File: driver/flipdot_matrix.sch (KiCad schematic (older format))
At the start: 45 parts, among them J2 CONN_02X32, Q1 DUAL_NPN_MOSFET, Q10 DUAL_NPN_MOSFET, Q11 DUAL_NPN_MOSFET, Q12 DUAL_NPN_MOSFET, Q13 DUAL_NPN_MOSFET, Q14 DUAL_NPN_MOSFET, Q15 DUAL_NPN_MOSFET, Q16 DUAL_NPN_MOSFET, Q17 DUAL_NPN_MOSFET, Q18 DUAL_NPN_MOSFET, Q19 DUAL_NPN_MOSFET, Q2 DUAL_NPN_MOSFET, Q20 DUAL_NPN_MOSFET, Q21 DUAL_NPN_MOSFET, Q22 DUAL_NPN_MOSFET, Q23 DUAL_NPN_MOSFET, Q24 DUAL_NPN_MOSFET, Q25 DUAL_NPN_MOSFET, Q26 DUAL_NPN_MOSFET, Q27 DUAL_NPN_MOSFET, Q28 DUAL_NPN_MOSFET, Q29 DUAL_NPN_MOSFET, Q3 DUAL_NPN_MOSFET, Q30 DUAL_NPN_MOSFET, Q31 DUAL_NPN_MOSFET, Q32 DUAL_NPN_MOSFET, Q33 DUAL_NPN_MOSFET, Q34 DUAL_NPN_MOSFET, Q35 DUAL_NPN_MOSFET, Q36 DUAL_NPN_MOSFET, Q37 DUAL_NPN_MOSFET, Q38 DUAL_NPN_MOSFET, Q39 DUAL_NPN_MOSFET, Q4 DUAL_NPN_MOSFET, Q40 DUAL_NPN_MOSFET, Q41 DUAL_NPN_MOSFET, Q42 DUAL_NPN_MOSFET, Q43 DUAL_NPN_MOSFET, Q44 DUAL_NPN_MOSFET, Q5 DUAL_NPN_MOSFET, Q6 DUAL_NPN_MOSFET, Q7 DUAL_NPN_MOSFET, Q8 DUAL_NPN_MOSFET, Q9 DUAL_NPN_MOSFET

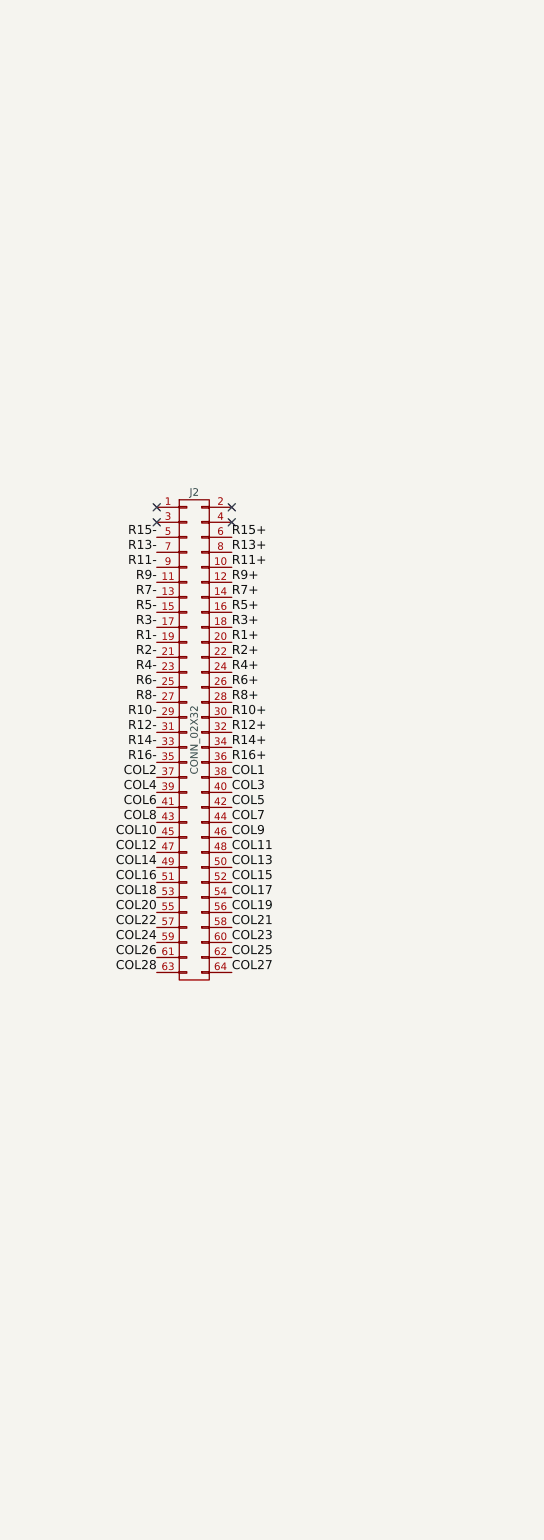
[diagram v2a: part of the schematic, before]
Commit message: wild changes
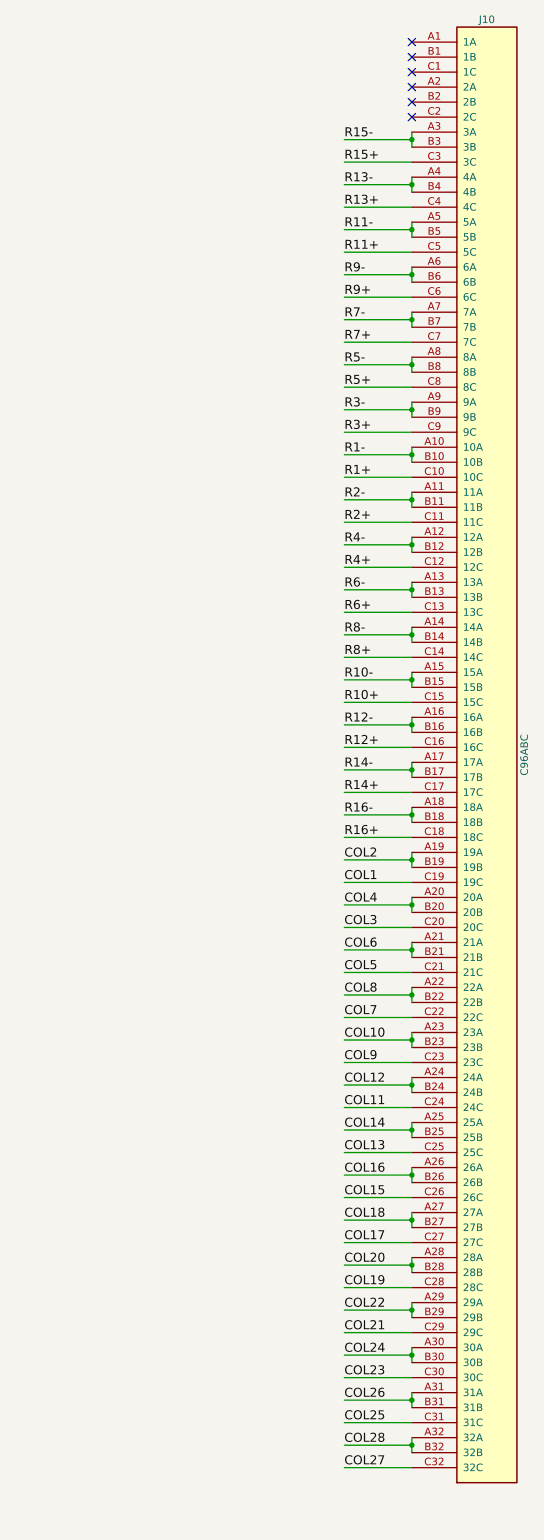
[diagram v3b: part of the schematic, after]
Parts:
- removed J2: CONN_02X32, Socket_Strips:Socket_Strip_Straight_2x32_Pitch2.54mm, symbol CONN_02X32
- added J10: C96ABC, Connectors:C96ABCMD, symbol C96ABC
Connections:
- net COL1: now also J10.C19 (19C)
- net COL10: now also J10.A23 (23A), J10.B23 (23B)
- net COL11: now also J10.C24 (24C)
- net COL12: now also J10.A24 (24A), J10.B24 (24B)
- net COL13: now also J10.C25 (25C)
- net COL14: now also J10.A25 (25A), J10.B25 (25B)
- net COL15: now also J10.C26 (26C)
- net COL16: now also J10.A26 (26A), J10.B26 (26B)
- net COL17: now also J10.C27 (27C)
- net COL18: now also J10.A27 (27A), J10.B27 (27B)
- net COL19: now also J10.C28 (28C)
- net COL2: now also J10.A19 (19A), J10.B19 (19B)
- net COL20: now also J10.A28 (28A), J10.B28 (28B)
- net COL21: now also J10.C29 (29C)
- net COL22: now also J10.A29 (29A), J10.B29 (29B)
- net COL23: now also J10.C30 (30C)
- net COL24: now also J10.A30 (30A), J10.B30 (30B)
- net COL25: now also J10.C31 (31C)
- net COL26: now also J10.A31 (31A), J10.B31 (31B)
- net COL27: now also J10.C32 (32C)
- net COL28: now also J10.A32 (32A), J10.B32 (32B)
- net COL3: now also J10.C20 (20C)
- net COL4: now also J10.A20 (20A), J10.B20 (20B)
- net COL5: now also J10.C21 (21C)
- net COL6: now also J10.A21 (21A), J10.B21 (21B)
- net COL7: now also J10.C22 (22C)
- net COL8: now also J10.A22 (22A), J10.B22 (22B)
- net COL9: now also J10.C23 (23C)
- net R1+: now also J10.C10 (10C)
- net R1-: now also J10.A10 (10A), J10.B10 (10B)
- net R10+: now also J10.C15 (15C)
- net R10-: now also J10.A15 (15A), J10.B15 (15B)
- net R11+: now also J10.C5 (5C)
- net R11-: now also J10.A5 (5A), J10.B5 (5B)
- net R12+: now also J10.C16 (16C)
- net R12-: now also J10.A16 (16A), J10.B16 (16B)
- net R13+: now also J10.C4 (4C)
- net R13-: now also J10.A4 (4A), J10.B4 (4B)
- net R14+: now also J10.C17 (17C)
- net R14-: now also J10.A17 (17A), J10.B17 (17B)
- net R15+: now also J10.C3 (3C)
- net R15-: now also J10.A3 (3A), J10.B3 (3B)
- net R16+: now also J10.C18 (18C)
- net R16-: now also J10.A18 (18A), J10.B18 (18B)
- net R2+: now also J10.C11 (11C)
- net R2-: now also J10.A11 (11A), J10.B11 (11B)
- net R3+: now also J10.C9 (9C)
- net R3-: now also J10.A9 (9A), J10.B9 (9B)
- net R4+: now also J10.C12 (12C)
- net R4-: now also J10.A12 (12A), J10.B12 (12B)
- net R5+: now also J10.C8 (8C)
- net R5-: now also J10.A8 (8A), J10.B8 (8B)
- net R6+: now also J10.C13 (13C)
- net R6-: now also J10.A13 (13A), J10.B13 (13B)
- net R7+: now also J10.C7 (7C)
- net R7-: now also J10.A7 (7A), J10.B7 (7B)
- net R8+: now also J10.C14 (14C)
- net R8-: now also J10.A14 (14A), J10.B14 (14B)
- net R9+: now also J10.C6 (6C)
- net R9-: now also J10.A6 (6A), J10.B6 (6B)
- no-connect marks 4 -> 6

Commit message: done??
probably not
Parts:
- J10: footprint Connectors:C96ABCMD -> img:C96ABCMD_custom
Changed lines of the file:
@@
 F 0 "J10" H 13000 10900 50  0000 C CNN
 F 1 "C96ABC" V 13250 6000 50  0000 C CNN
-F 2 "Connectors:C96ABCMD" H 13000 6000 50  0001 C CNN
+F 2 "img:C96ABCMD_custom" H 13000 6000 50  0001 C CNN
 F 3 "" H 13000 6000 50  0001 C CNN
 	1    13000 6000

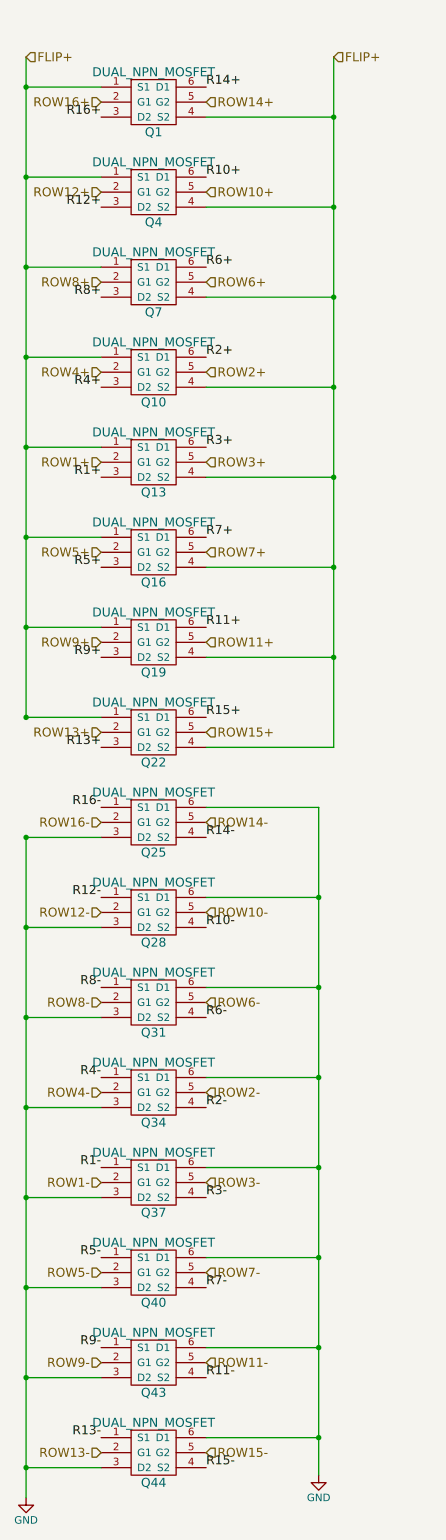
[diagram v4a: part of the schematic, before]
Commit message: fix major goof
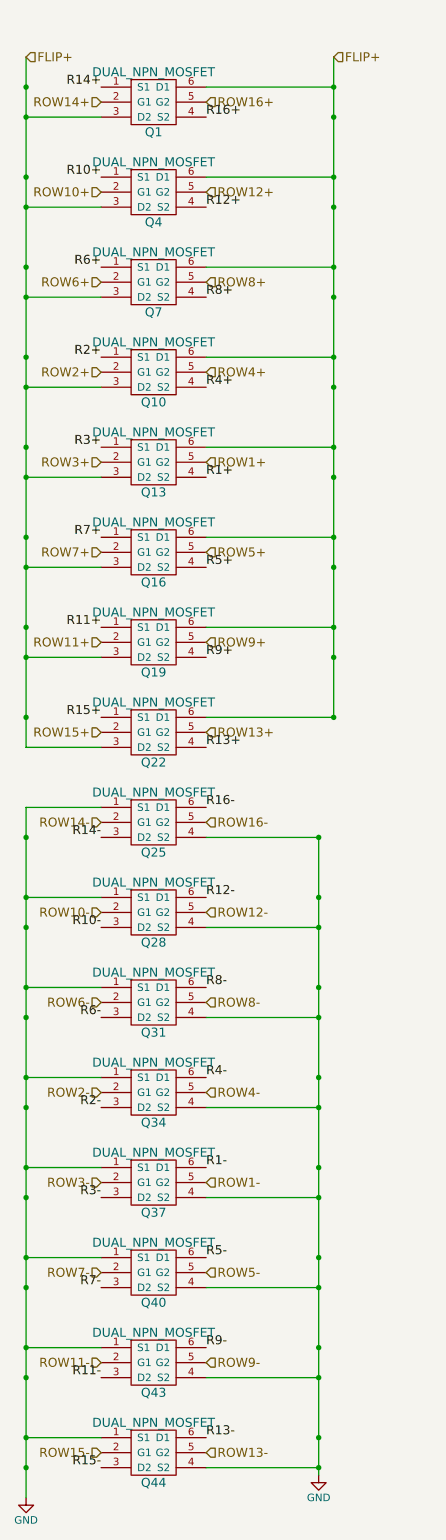
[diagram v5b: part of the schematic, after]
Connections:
- net FLIP+: now also Q1.3 (D2), Q1.6 (D1), Q10.3 (D2), Q10.6 (D1), Q13.3 (D2), Q13.6 (D1), Q16.3 (D2), Q16.6 (D1), Q19.3 (D2), Q19.6 (D1), Q22.3 (D2), Q22.6 (D1), Q4.3 (D2), Q4.6 (D1), Q7.3 (D2), Q7.6 (D1); no longer Q1.1 (S1), Q1.4 (S2), Q10.1 (S1), Q10.4 (S2), Q13.1 (S1), Q13.4 (S2), Q16.1 (S1), Q16.4 (S2), Q19.1 (S1), Q19.4 (S2), Q22.1 (S1), Q22.4 (S2), Q4.1 (S1), Q4.4 (S2), Q7.1 (S1), Q7.4 (S2)
- net GND: now also Q25.1 (S1), Q25.4 (S2), Q28.1 (S1), Q28.4 (S2), Q31.1 (S1), Q31.4 (S2), Q34.1 (S1), Q34.4 (S2), Q37.1 (S1), Q37.4 (S2), Q40.1 (S1), Q40.4 (S2), Q43.1 (S1), Q43.4 (S2), Q44.1 (S1), Q44.4 (S2); no longer Q25.3 (D2), Q25.6 (D1), Q28.3 (D2), Q28.6 (D1), Q31.3 (D2), Q31.6 (D1), Q34.3 (D2), Q34.6 (D1), Q37.3 (D2), Q37.6 (D1), Q40.3 (D2), Q40.6 (D1), Q43.3 (D2), Q43.6 (D1), Q44.3 (D2), Q44.6 (D1)
- net R1+: now also Q13.4 (S2); no longer Q13.3 (D2)
- net R1-: now also Q37.6 (D1); no longer Q37.1 (S1)
- net R10+: now also Q4.1 (S1); no longer Q4.6 (D1)
- net R10-: now also Q28.3 (D2); no longer Q28.4 (S2)
- net R11+: now also Q19.1 (S1); no longer Q19.6 (D1)
- net R11-: now also Q43.3 (D2); no longer Q43.4 (S2)
- net R12+: now also Q4.4 (S2); no longer Q4.3 (D2)
- net R12-: now also Q28.6 (D1); no longer Q28.1 (S1)
- net R13+: now also Q22.4 (S2); no longer Q22.3 (D2)
- net R13-: now also Q44.6 (D1); no longer Q44.1 (S1)
- net R14+: now also Q1.1 (S1); no longer Q1.6 (D1)
- net R14-: now also Q25.3 (D2); no longer Q25.4 (S2)
- net R15+: now also Q22.1 (S1); no longer Q22.6 (D1)
- net R15-: now also Q44.3 (D2); no longer Q44.4 (S2)
- net R16+: now also Q1.4 (S2); no longer Q1.3 (D2)
- net R16-: now also Q25.6 (D1); no longer Q25.1 (S1)
- net R2+: now also Q10.1 (S1); no longer Q10.6 (D1)
- net R2-: now also Q34.3 (D2); no longer Q34.4 (S2)
- net R3+: now also Q13.1 (S1); no longer Q13.6 (D1)
- net R3-: now also Q37.3 (D2); no longer Q37.4 (S2)
- net R4+: now also Q10.4 (S2); no longer Q10.3 (D2)
- net R4-: now also Q34.6 (D1); no longer Q34.1 (S1)
- net R5+: now also Q16.4 (S2); no longer Q16.3 (D2)
- net R5-: now also Q40.6 (D1); no longer Q40.1 (S1)
- net R6+: now also Q7.1 (S1); no longer Q7.6 (D1)
- net R6-: now also Q31.3 (D2); no longer Q31.4 (S2)
- net R7+: now also Q16.1 (S1); no longer Q16.6 (D1)
- net R7-: now also Q40.3 (D2); no longer Q40.4 (S2)
- net R8+: now also Q7.4 (S2); no longer Q7.3 (D2)
- net R8-: now also Q31.6 (D1); no longer Q31.1 (S1)
- net R9+: now also Q19.4 (S2); no longer Q19.3 (D2)
- net R9-: now also Q43.6 (D1); no longer Q43.1 (S1)
- net ROW1+: now also Q13.5 (G2); no longer Q13.2 (G1)
- net ROW1-: now also Q37.5 (G2); no longer Q37.2 (G1)
- net ROW10+: now also Q4.2 (G1); no longer Q4.5 (G2)
- net ROW10-: now also Q28.2 (G1); no longer Q28.5 (G2)
- net ROW11+: now also Q19.2 (G1); no longer Q19.5 (G2)
- net ROW11-: now also Q43.2 (G1); no longer Q43.5 (G2)
- net ROW12+: now also Q4.5 (G2); no longer Q4.2 (G1)
- net ROW12-: now also Q28.5 (G2); no longer Q28.2 (G1)
- net ROW13+: now also Q22.5 (G2); no longer Q22.2 (G1)
- net ROW13-: now also Q44.5 (G2); no longer Q44.2 (G1)
- net ROW14+: now also Q1.2 (G1); no longer Q1.5 (G2)
- net ROW14-: now also Q25.2 (G1); no longer Q25.5 (G2)
- net ROW15+: now also Q22.2 (G1); no longer Q22.5 (G2)
- net ROW15-: now also Q44.2 (G1); no longer Q44.5 (G2)
- net ROW16+: now also Q1.5 (G2); no longer Q1.2 (G1)
- net ROW16-: now also Q25.5 (G2); no longer Q25.2 (G1)
- net ROW2+: now also Q10.2 (G1); no longer Q10.5 (G2)
- net ROW2-: now also Q34.2 (G1); no longer Q34.5 (G2)
- net ROW3+: now also Q13.2 (G1); no longer Q13.5 (G2)
- net ROW3-: now also Q37.2 (G1); no longer Q37.5 (G2)
- net ROW4+: now also Q10.5 (G2); no longer Q10.2 (G1)
- net ROW4-: now also Q34.5 (G2); no longer Q34.2 (G1)
- net ROW5+: now also Q16.5 (G2); no longer Q16.2 (G1)
- net ROW5-: now also Q40.5 (G2); no longer Q40.2 (G1)
- net ROW6+: now also Q7.2 (G1); no longer Q7.5 (G2)
- net ROW6-: now also Q31.2 (G1); no longer Q31.5 (G2)
- net ROW7+: now also Q16.2 (G1); no longer Q16.5 (G2)
- net ROW7-: now also Q40.2 (G1); no longer Q40.5 (G2)
- net ROW8+: now also Q7.5 (G2); no longer Q7.2 (G1)
- net ROW8-: now also Q31.5 (G2); no longer Q31.2 (G1)
- net ROW9+: now also Q19.5 (G2); no longer Q19.2 (G1)
- net ROW9-: now also Q43.5 (G2); no longer Q43.2 (G1)
